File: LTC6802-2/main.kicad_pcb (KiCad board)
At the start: 2 copper layers, 50.8 x 40.6 mm, 10 parts, among them P1 CONN_01X13, P2 CONN_01X04, P3 CONN_01X04, P4 CONN_01X06, P5 CONN_01X13, U1 LTC6802-2

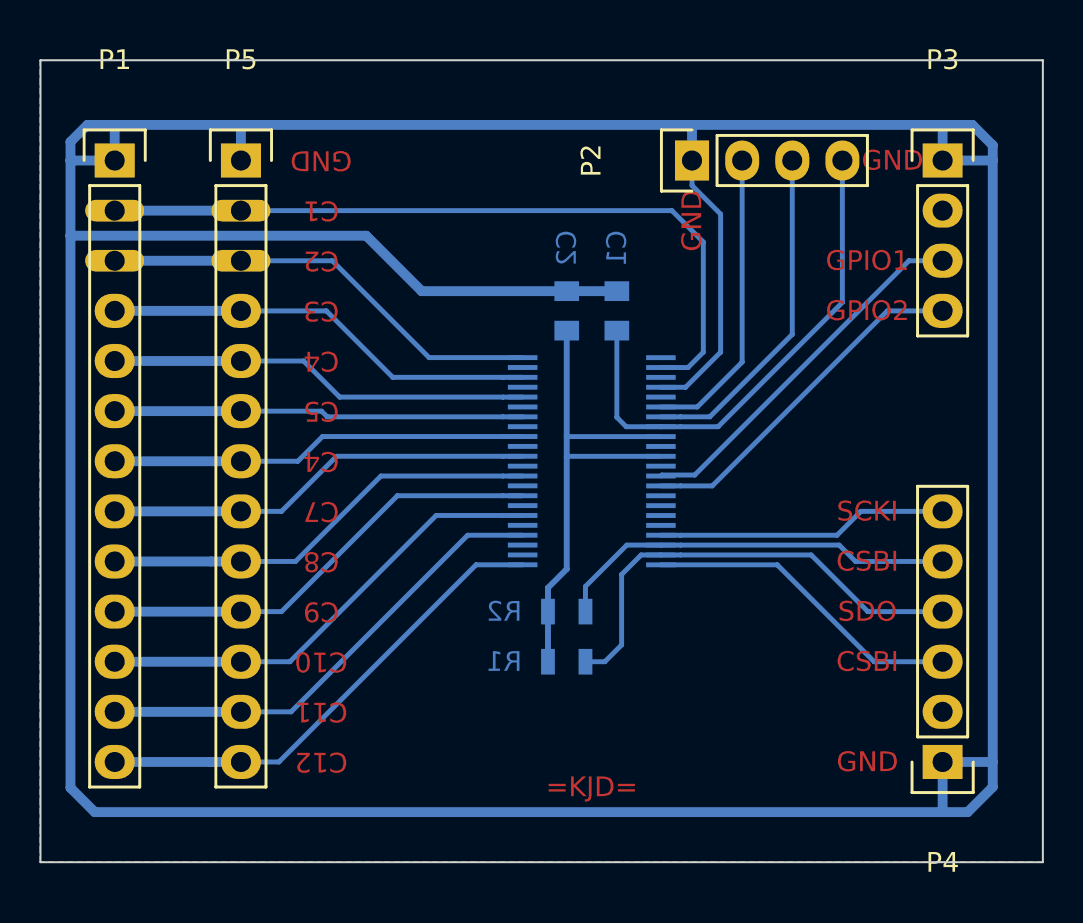
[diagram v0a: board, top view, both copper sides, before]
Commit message: test
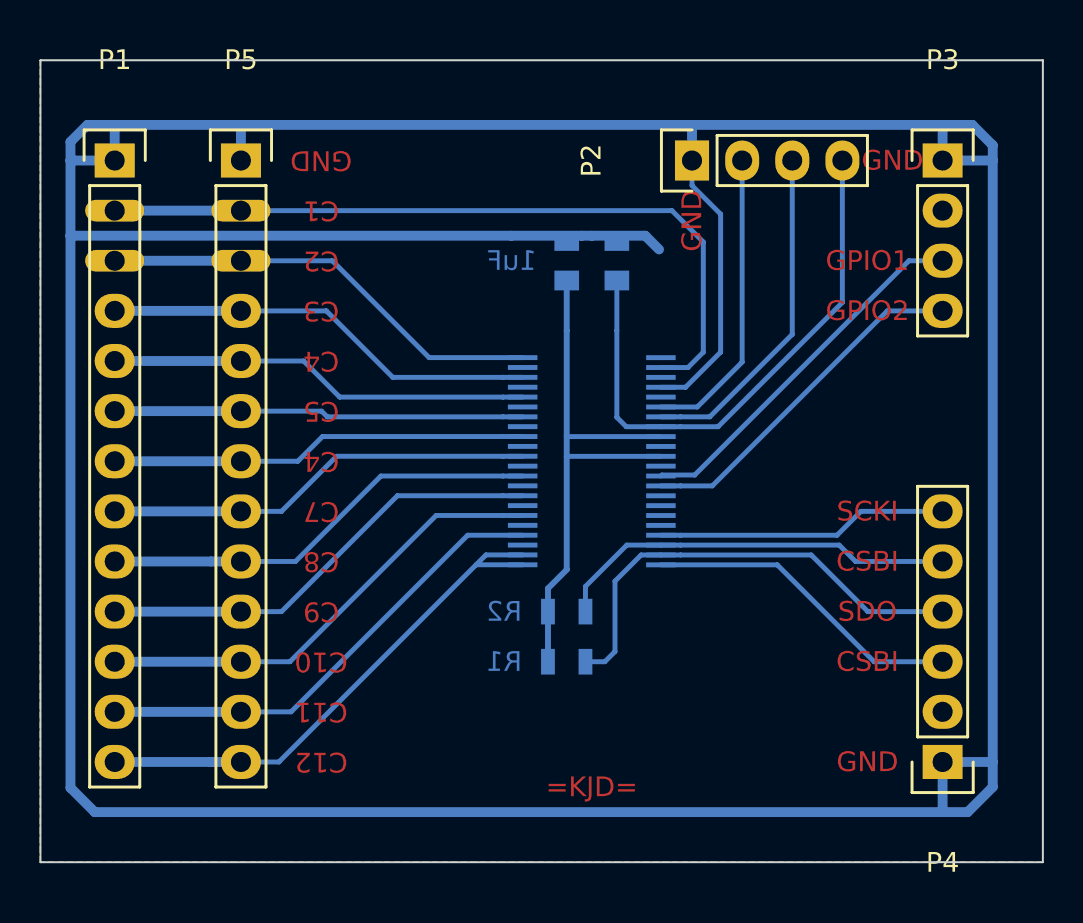
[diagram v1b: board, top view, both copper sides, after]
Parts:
- moved C1 2.54 mm to (148.6, 109.2)
- moved C2 2.54 mm to (146.1, 109.2)
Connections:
- net Net-(P2-Pad2) renamed /Vtemp1
- net Net-(P2-Pad3) renamed /Vtemp2
- P4 pad 5: /CSBI -> /SDI
- R2 pad 1: /CSBI -> /SDI
- U1 pad 42: /CSBI -> /SDI
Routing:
- net /CSBI: track 36.9 -> 16.3 mm
- net /SDI: track 0.00 -> 20.6 mm
- net GND: track 221.4 -> 224.6 mm
- net /C12: track 24.8 -> 27.4 mm
- net Net-(C1-Pad2): track 25.8 -> 28.4 mm
- net +5V: track 26.7 -> 29.3 mm
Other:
- board text added: "1uF"
